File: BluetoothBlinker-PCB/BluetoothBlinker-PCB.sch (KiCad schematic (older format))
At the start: 51 parts, among them J1 USB_C_Receptacle_USB2.0, J2 Programming Connector, J3 Expansion Header, SW1 SW_Push, U1 CH340E, U2 TLV75533PDBV, U3 CC2642R, Y1 48MHz, Y2 32.768kHz

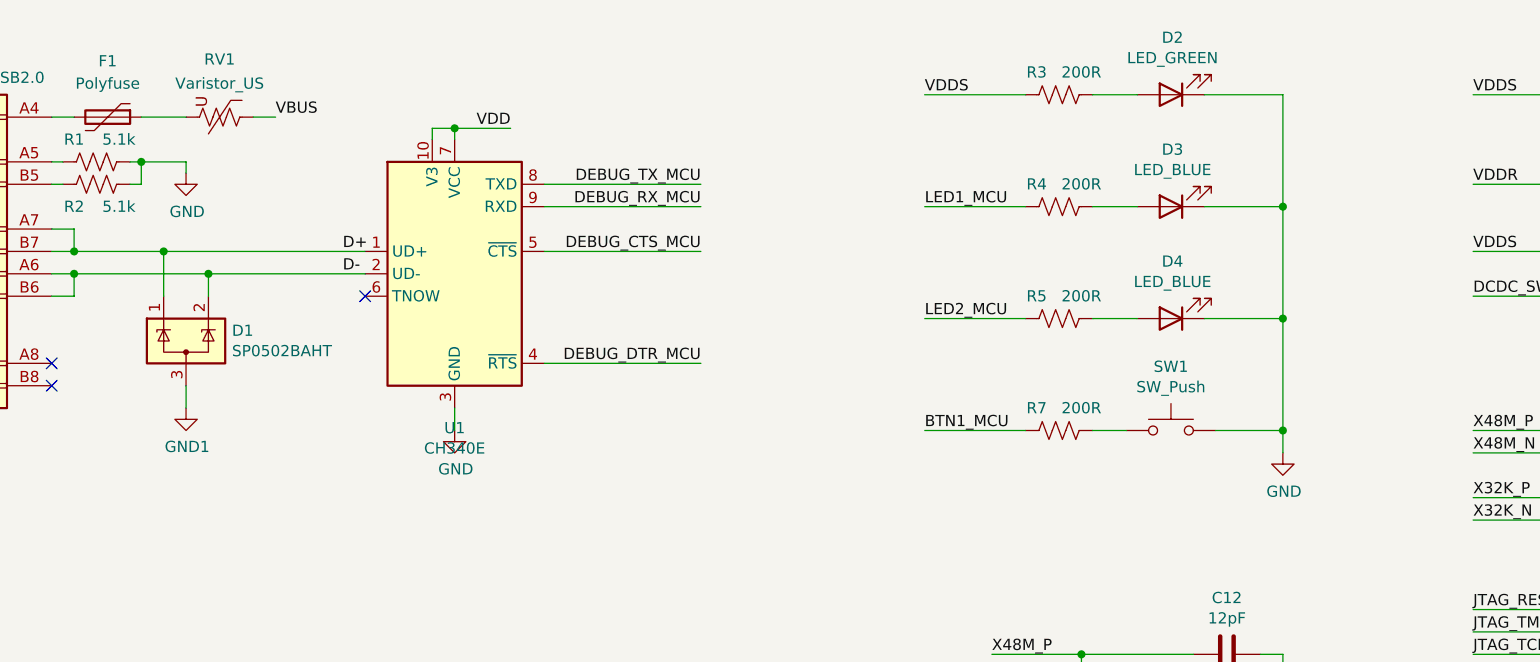
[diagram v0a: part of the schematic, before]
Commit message: Minor updates
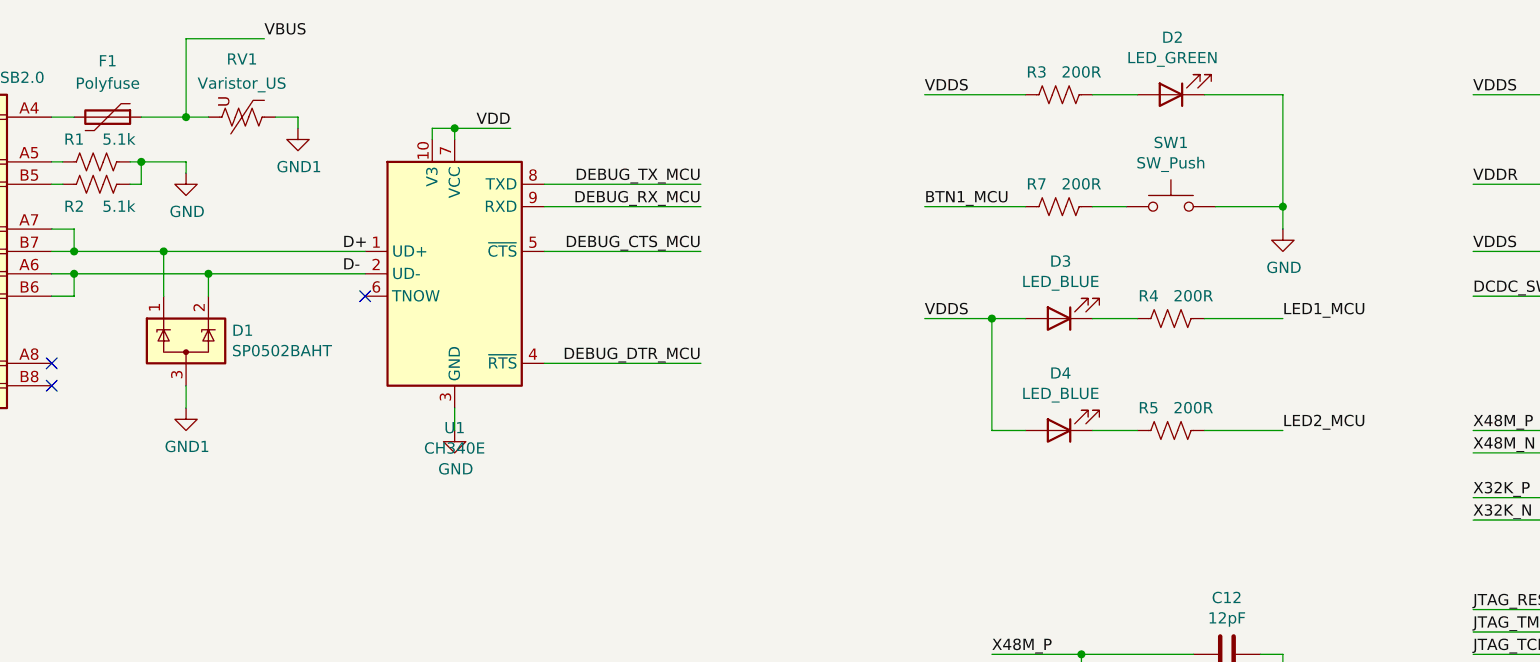
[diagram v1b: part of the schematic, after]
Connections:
- net GND: no longer D3.1 (K), D4.1 (K)
- net GND1: now also RV1.1
- net LED1_MCU: now also R4.2; no longer R4.1
- net LED2_MCU: now also R5.2; no longer R5.1
- net VBUS: now also F1.1, RV1.2; no longer RV1.1
- net VDDS: now also D3.2 (A), D4.2 (A)
- new net: D3.1 (K), R4.1
- new net: D4.1 (K), R5.1
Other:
- moved on the sheet: D3, D4, R4, R5, R7, RV1, SW1
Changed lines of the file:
@@
 Wire Wire Line
 	2600 2400 2600 2300
-$Comp
-L Device:Varistor_US RV1
-U 1 1 5FDD0C56
-P 2750 1100
-F 0 "RV1" V 2492 1100 50  0000 C CNN
-F 1 "Varistor_US" V 2600 1100 50  0000 C CNN
-F 2 "Resistor_SMD:R_0603_1608Metric" V 2680 1100 50  0001 C CNN
-F 3 "https://www.littelfuse.com/products/varistors/multilayer/mla/v5_5mla0603.aspx" H 2750 1100 50  0001 C CNN
-	1    2750 1100
-	0    1    1    0
-$EndComp
 Wire Wire Line
 	2100 1100 2000 1100
-Text Label 3000 1100 0    50   ~ 0
+Text Label 2950 750  0    50   ~ 0
 VBUS
-Wire Wire Line
-	3000 1100 2900 1100
-$Comp
-L Device:Polyfuse F1
-U 1 1 5FDFAF4B
-P 2250 1100
-F 0 "F1" V 2000 1100 50  0000 C CNN
-F 1 "Polyfuse" V 2100 1100 50  0000 C CNN
-F 2 "Resistor_SMD:R_1206_3216Metric" H 2300 900 50  0001 L CNN
-F 3 "https://www.littelfuse.com/~/media/electronics/datasheets/resettable_ptcs/littelfuse_ptc_low_rho_datasheet.pdf.pdf" H 2250 1100 50  0001 C CNN
-F 4 "1206L150SL" V 2250 1100 50  0001 C CNN "Device"
-	1    2250 1100
-	0    1    1    0
-$EndComp
 Wire Wire Line
 	2400 1100 2600 1100
@@
 L Device:LED D3
 U 1 1 60955642
-P 7000 1500
-F 0 "D3" H 6993 1245 50  0000 C CNN
-F 1 "LED_BLUE" H 6993 1336 50  0000 C CNN
-F 2 "LED_SMD:LED_0603_1608Metric" H 7000 1500 50  0001 C CNN
-F 3 "https://www.kingbrightusa.com/images/catalog/SPEC/APT3216QBC-D.pdf" H 7000 1500 50  0001 C CNN
-	1    7000 1500
+P 6500 2000
+F 0 "D3" H 6493 1745 50  0000 C CNN
+F 1 "LED_BLUE" H 6493 1836 50  0000 C CNN
+F 2 "LED_SMD:LED_0603_1608Metric" H 6500 2000 50  0001 C CNN
+F 3 "https://www.kingbrightusa.com/images/catalog/SPEC/APT3216QBC-D.pdf" H 6500 2000 50  0001 C CNN
+	1    6500 2000
 	-1   0    0    1
 $EndComp
@@
 L Device:R_US R4
 U 1 1 609814AB
-P 6500 1500
-F 0 "R4" V 6600 1600 50  0000 C CNN
-F 1 "200R" V 6600 1400 50  0000 C CNN
-F 2 "Resistor_SMD:R_0603_1608Metric" V 6540 1490 50  0001 C CNN
-F 3 "~" H 6500 1500 50  0001 C CNN
-	1    6500 1500
+P 7000 2000
+F 0 "R4" V 7100 2100 50  0000 C CNN
+F 1 "200R" V 7100 1900 50  0000 C CNN
+F 2 "Resistor_SMD:R_0603_1608Metric" V 7040 1990 50  0001 C CNN
+F 3 "~" H 7000 2000 50  0001 C CNN
+	1    7000 2000
 	0    -1   -1   0
 $EndComp
@@
 L Device:R_US R5
 U 1 1 60981A2C
-P 6500 2000
-F 0 "R5" V 6600 2100 50  0000 C CNN
-F 1 "200R" V 6600 1900 50  0000 C CNN
-F 2 "Resistor_SMD:R_0603_1608Metric" V 6540 1990 50  0001 C CNN
-F 3 "~" H 6500 2000 50  0001 C CNN
-	1    6500 2000
+P 7000 2500
+F 0 "R5" V 7100 2600 50  0000 C CNN
+F 1 "200R" V 7100 2400 50  0000 C CNN
+F 2 "Resistor_SMD:R_0603_1608Metric" V 7040 2490 50  0001 C CNN
+F 3 "~" H 7000 2500 50  0001 C CNN
+	1    7000 2500
 	0    -1   -1   0
 $EndComp
@@
 VDDS
 Wire Wire Line
+	6650 2500 6850 2500
+Wire Wire Line
 	6650 2000 6850 2000
-Wire Wire Line
-	6650 1500 6850 1500
 Wire Wire Line
 	6850 1000 6650 1000
@@
 L power:GND #PWR01
 U 1 1 6005E763
-P 7500 2600
-F 0 "#PWR01" H 7500 2350 50  0001 C CNN
-F 1 "GND" H 7505 2427 50  0000 C CNN
-F 2 "" H 7500 2600 50  0001 C CNN
-F 3 "" H 7500 2600 50  0001 C CNN
-	1    7500 2600
+P 7500 1600
+F 0 "#PWR01" H 7500 1350 50  0001 C CNN
+F 1 "GND" H 7505 1427 50  0000 C CNN
+F 2 "" H 7500 1600 50  0001 C CNN
+F 3 "" H 7500 1600 50  0001 C CNN
+	1    7500 1600
 	1    0    0    -1
 $EndComp
@@
 	7500 1000 7150 1000
 Wire Wire Line
-	7500 1000 7500 1500
-Connection ~ 7500 2000
-Wire Wire Line
-	7500 1500 7150 1500
-Connection ~ 7500 1500
-Wire Wire Line
-	7500 1500 7500 2000
-Text Label 5900 1500 0    50   ~ 0
+	7500 2000 7150 2000
+Text Label 7500 2000 0    50   ~ 0
 LED1_MCU
-Text Label 5900 2000 0    50   ~ 0
+Text Label 7500 2500 0    50   ~ 0
 LED2_MCU
 Wire Wire Line
-	5900 2000 6350 2000
-Wire Wire Line
-	5900 1500 6350 1500
+	5900 2000 6200 2000
 Wire Wire Line
 	5900 1000 6350 1000
@@
 $EndComp
 Wire Wire Line
-	7500 2000 7150 2000
+	7500 2500 7150 2500
 $Comp
 L Device:LED D4
 U 1 1 609562A4
-P 7000 2000
-F 0 "D4" H 6993 1745 50  0000 C CNN
-F 1 "LED_BLUE" H 6993 1836 50  0000 C CNN
-F 2 "LED_SMD:LED_0603_1608Metric" H 7000 2000 50  0001 C CNN
-F 3 "https://www.kingbrightusa.com/images/catalog/SPEC/APT3216QBC-D.pdf" H 7000 2000 50  0001 C CNN
-	1    7000 2000
+P 6500 2500
+F 0 "D4" H 6493 2245 50  0000 C CNN
+F 1 "LED_BLUE" H 6493 2336 50  0000 C CNN
+F 2 "LED_SMD:LED_0603_1608Metric" H 6500 2500 50  0001 C CNN
+F 3 "https://www.kingbrightusa.com/images/catalog/SPEC/APT3216QBC-D.pdf" H 6500 2500 50  0001 C CNN
+	1    6500 2500
 	-1   0    0    1
 $EndComp
 Wire Wire Line
-	7500 2000 7500 2500
-Wire Wire Line
-	7500 2500 7200 2500
-Connection ~ 7500 2500
-Wire Wire Line
-	7500 2500 7500 2600
-Text Label 5900 2500 0    50   ~ 0
+	7500 1500 7200 1500
+Text Label 5900 1500 0    50   ~ 0
 BTN1_MCU
 Wire Wire Line
-	5900 2500 6350 2500
+	5900 1500 6350 1500
 $Comp
 L Device:R_US R7
 U 1 1 6022C1CA
-P 6500 2500
-F 0 "R7" V 6600 2600 50  0000 C CNN
-F 1 "200R" V 6600 2400 50  0000 C CNN
-F 2 "Resistor_SMD:R_0603_1608Metric" V 6540 2490 50  0001 C CNN
-F 3 "~" H 6500 2500 50  0001 C CNN
-	1    6500 2500
+P 6500 1500
+F 0 "R7" V 6600 1600 50  0000 C CNN
+F 1 "200R" V 6600 1400 50  0000 C CNN
+F 2 "Resistor_SMD:R_0603_1608Metric" V 6540 1490 50  0001 C CNN
+F 3 "~" H 6500 1500 50  0001 C CNN
+	1    6500 1500
 	0    -1   -1   0
 $EndComp
 Wire Wire Line
-	6650 2500 6800 2500
+	6650 1500 6800 1500
 $Comp
 L BluetoothBlinker-PCB-rescue:Antenna-Device AE1
@@
 L Switch:SW_Push SW1
 U 1 1 601EE08E
-P 7000 2500
-F 0 "SW1" H 7000 2785 50  0000 C CNN
-F 1 "SW_Push" H 7000 2694 50  0000 C CNN
-F 2 "Button_Switch_THT:SW_PUSH_6mm" H 7000 2700 50  0001 C CNN
-F 3 "https://datasheet.octopart.com/TL3305AF160QG-E-Switch-datasheet-100437264.pdf" H 7000 2700 50  0001 C CNN
-	1    7000 2500
+P 7000 1500
+F 0 "SW1" H 7000 1785 50  0000 C CNN
+F 1 "SW_Push" H 7000 1694 50  0000 C CNN
+F 2 "Button_Switch_THT:SW_PUSH_6mm" H 7000 1700 50  0001 C CNN
+F 3 "https://datasheet.octopart.com/TL3305AF160QG-E-Switch-datasheet-100437264.pdf" H 7000 1700 50  0001 C CNN
+	1    7000 1500
 	1    0    0    -1
 $EndComp
@@
 Wire Wire Line
 	2700 1800 3400 1800
+Wire Wire Line
+	2600 750  2950 750
+Wire Wire Line
+	2600 750  2600 1100
+Wire Wire Line
+	2700 1100 2600 1100
+Connection ~ 2600 1100
+$Comp
+L power:GND1 #PWR0116
+U 1 1 60E8327C
+P 3100 1150
+F 0 "#PWR0116" H 3100 900 50  0001 C CNN
+F 1 "GND1" H 3105 977 50  0000 C CNN
+F 2 "" H 3100 1150 50  0001 C CNN
+F 3 "" H 3100 1150 50  0001 C CNN
+	1    3100 1150
+	1    0    0    -1
+$EndComp
+Wire Wire Line
+	3000 1100 3100 1100
+Wire Wire Line
+	3100 1100 3100 1150
+Wire Wire Line
+	7500 1000 7500 1500
+Wire Wire Line
+	7500 1600 7500 1500
+Connection ~ 7500 1500
+Wire Wire Line
+	6200 2500 6200 2000
+Wire Wire Line
+	6200 2500 6350 2500
+Connection ~ 6200 2000
+Wire Wire Line
+	6200 2000 6350 2000
+Text Label 5900 2000 0    50   ~ 0
+VDDS
+$Comp
+L Device:Varistor_US RV1
+U 1 1 5FDD0C56
+P 2850 1100
+F 0 "RV1" V 2592 1100 50  0000 C CNN
+F 1 "Varistor_US" V 2700 1100 50  0000 C CNN
+F 2 "Resistor_SMD:R_0603_1608Metric" V 2780 1100 50  0001 C CNN
+F 3 "https://www.littelfuse.com/products/varistors/multilayer/mla/v5_5mla0603.aspx" H 2850 1100 50  0001 C CNN
+	1    2850 1100
+	0    1    1    0
+$EndComp
+$Comp
+L Device:Polyfuse F1
+U 1 1 5FDFAF4B
+P 2250 1100
+F 0 "F1" V 2000 1100 50  0000 C CNN
+F 1 "Polyfuse" V 2100 1100 50  0000 C CNN
+F 2 "Resistor_SMD:R_1206_3216Metric" H 2300 900 50  0001 L CNN
+F 3 "https://www.littelfuse.com/~/media/electronics/datasheets/resettable_ptcs/littelfuse_ptc_low_rho_datasheet.pdf.pdf" H 2250 1100 50  0001 C CNN
+F 4 "1206L150SL" V 2250 1100 50  0001 C CNN "Device"
+	1    2250 1100
+	0    1    1    0
+$EndComp
 $EndSCHEMATC
